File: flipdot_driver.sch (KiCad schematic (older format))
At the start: 0 parts

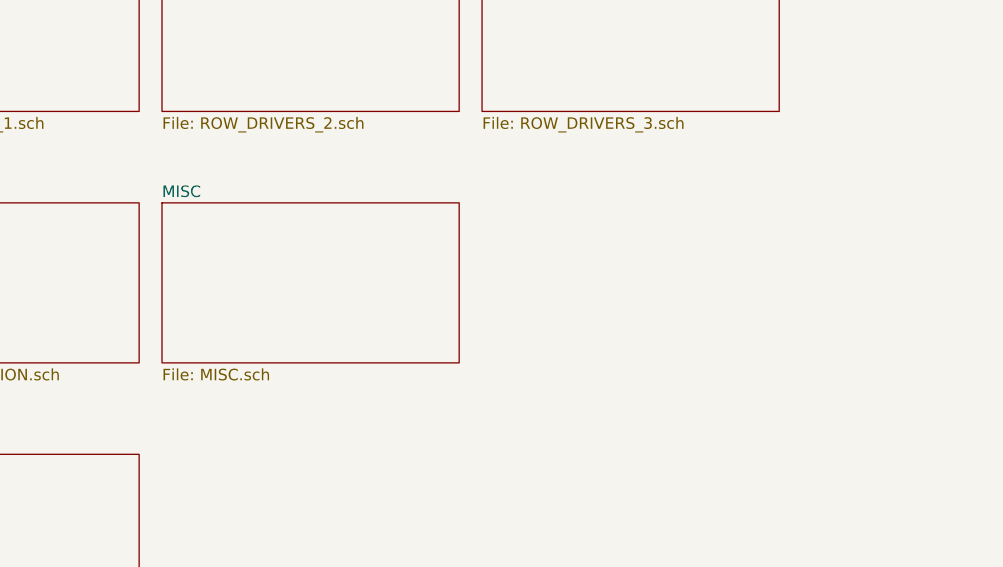
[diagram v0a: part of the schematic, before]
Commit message: automated commit
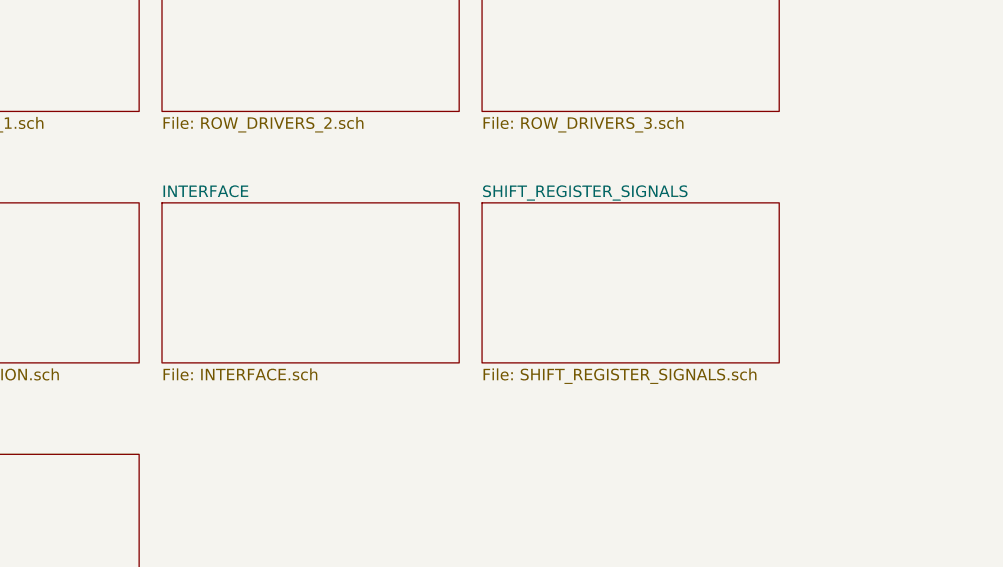
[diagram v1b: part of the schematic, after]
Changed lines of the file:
@@
 $Descr A4 11693 8268
 encoding utf-8
-Sheet 1 19
+Sheet 1 20
 Title ""
 Date ""
@@
 S 3600 3200 1300 700
 U 627E3ADC
-F0 "MISC" 50
-F1 "MISC.sch" 50
+F0 "INTERFACE" 50
+F1 "INTERFACE.sch" 50
 $EndSheet
 $Sheet
@@
 F1 "ROW_DRIVERS_3.sch" 50
 $EndSheet
+$Sheet
+S 5000 3200 1300 700
+U 5D4A63FF
+F0 "SHIFT_REGISTER_SIGNALS" 50
+F1 "SHIFT_REGISTER_SIGNALS.sch" 50
+$EndSheet
 $EndSCHEMATC
